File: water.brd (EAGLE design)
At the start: 100 x 80 mm, 15 parts, among them K1 AQH2223, K2 AQH2223, K3 AQH2223, K4 AQH2223, X5 MKDSN1,5/2-5,08, X6 MKDSN1,5/2-5,08, X7 MKDSN1,5/2-5,08, X8 MKDSN1,5/2-5,08

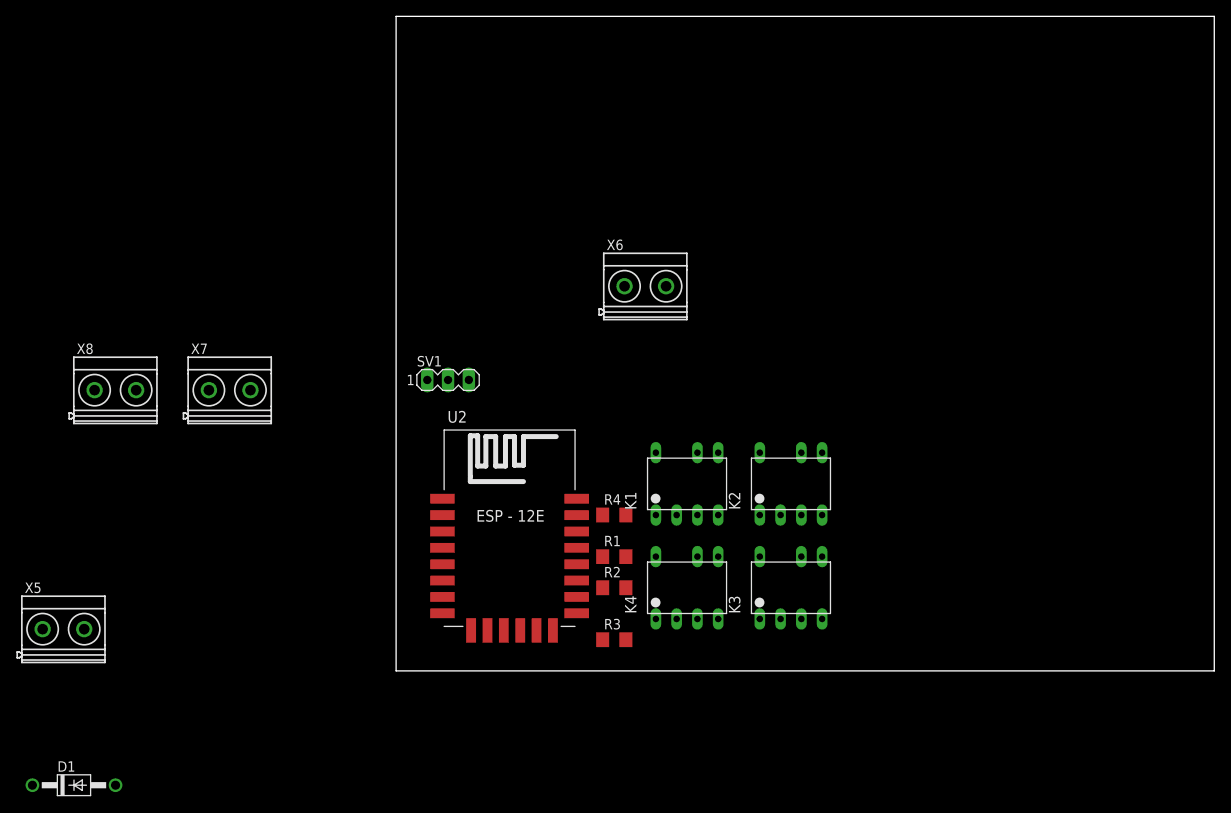
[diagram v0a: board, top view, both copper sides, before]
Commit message: Changes
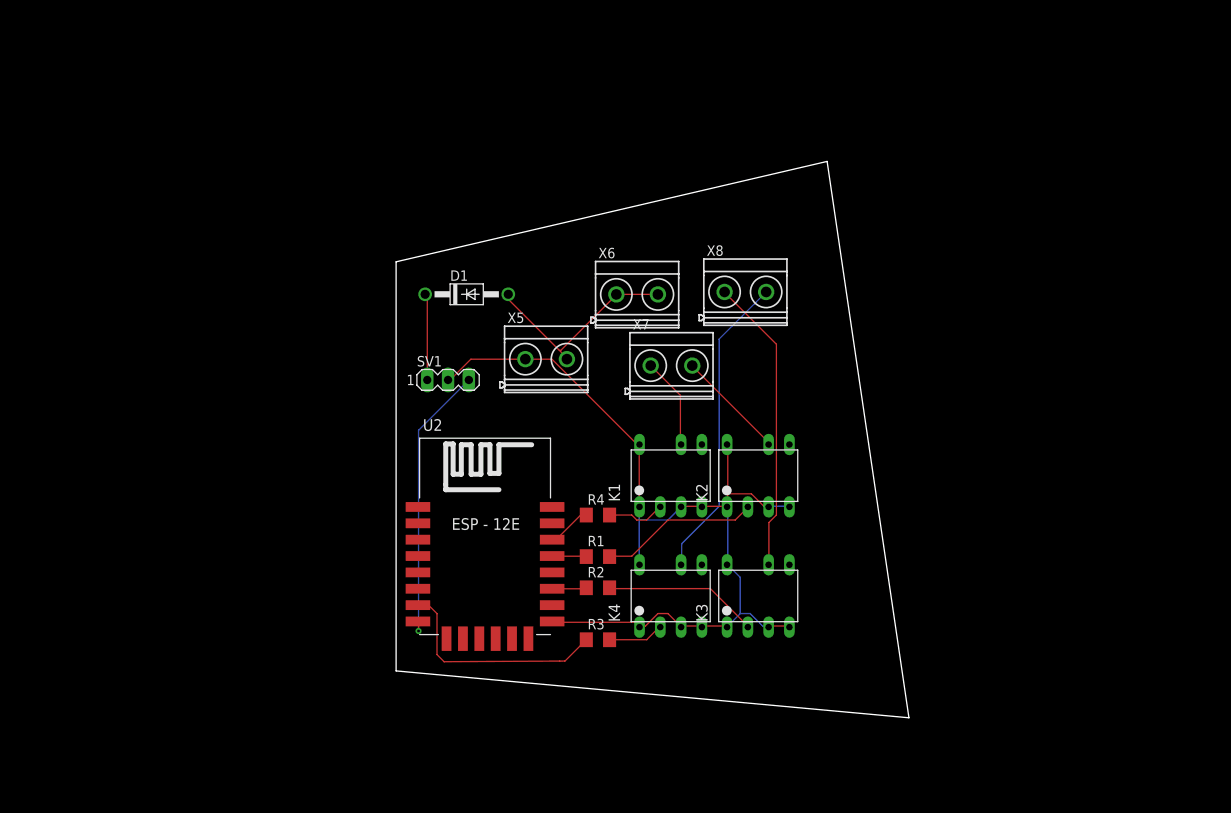
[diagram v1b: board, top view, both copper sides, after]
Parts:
- moved X8 77.9 mm to (42.7, 46.3)
- moved D1 76.8 mm to (8.63, 46.0)
- moved X5 67.6 mm to (18.4, 38.1)
- moved X7 54.1 mm to (33.7, 37.3)
- moved K2 4.12 mm to (44.3, 23.9)
- moved K3 4.12 mm to (44.3, 9.16)
- moved U2 3.16 mm to (11.0, 14.2)
- moved K1 2.24 mm to (33.6, 23.9)
- moved K4 2.24 mm to (33.6, 9.16)
- moved R1 2.00 mm to (24.7, 14.0)
- moved R2 2.00 mm to (24.7, 10.2)
- moved R3 2.00 mm to (24.7, 3.81)
- moved R4 2.00 mm to (24.7, 19.1)
- moved X6 1.41 mm to (29.5, 46.0)
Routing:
- net GND: track 0.00 -> 117.8 mm
- net N$9: track 0.00 -> 37.6 mm
- net N$10: track 0.00 -> 36.3 mm
- net +3V3: track 0.00 -> 34.4 mm, vias 0 -> 1
- net N$8: track 0.00 -> 27.5 mm
- net N$15: track 0.00 -> 25.8 mm
- net N$2: track 0.00 -> 19.4 mm
- net N$3: track 0.00 -> 19.0 mm
- net N$11: track 0.00 -> 13.5 mm
- net N$12: track 0.00 -> 11.2 mm
- net N$14: track 0.00 -> 10.6 mm
- net N$1: track 0.00 -> 7.11 mm
- net N$4: track 0.00 -> 6.83 mm
- net N$5: track 0.00 -> 5.42 mm
- net N$7: track 0.00 -> 4.23 mm
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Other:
- board size 100 x 80 mm -> 62.7 x 68 mm

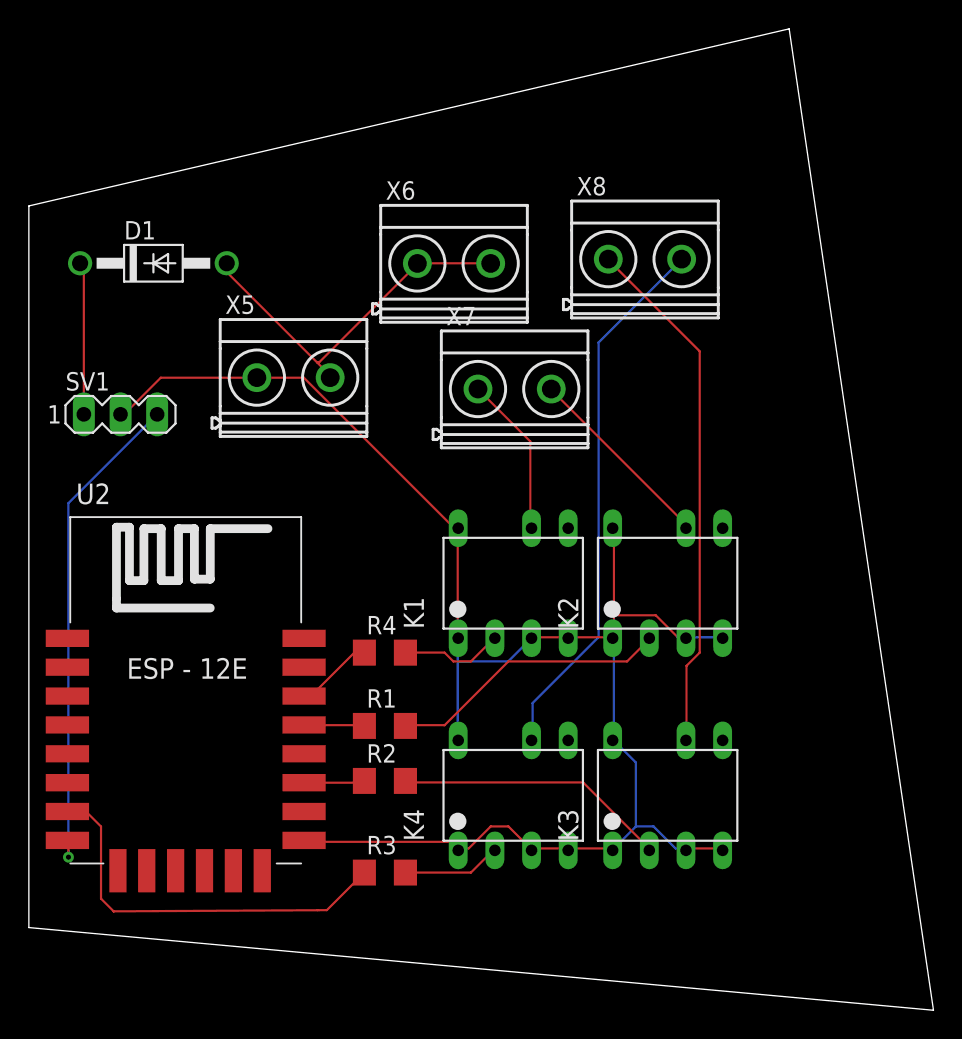
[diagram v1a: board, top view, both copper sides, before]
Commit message: Move parts
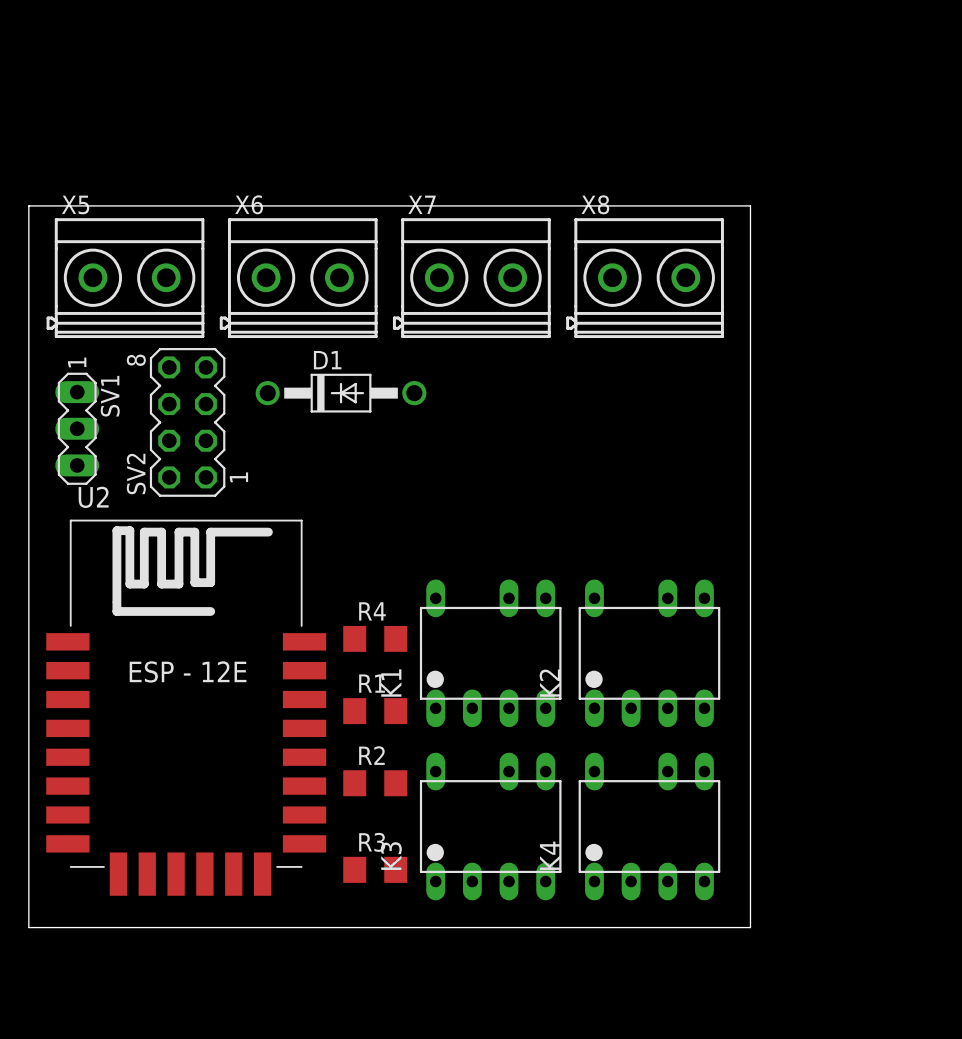
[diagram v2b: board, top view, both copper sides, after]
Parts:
- added SV2: (no value), con-lstb:MA04-2
- R1, R2, R3, R4: value 220 -> (none)
- moved D1 15.8 mm to (21.6, 37.0)
- moved X5 13.3 mm to (7.00, 45.0)
- moved K3 12.4 mm to (32.0, 7.00)
- moved X6 10.5 mm to (19.0, 45.0)
- moved K4 9.68 mm to (43.0, 7.00)
- moved X7 8.16 mm to (31.0, 45.0)
- moved K1 5.10 mm to (32.0, 19.0)
- moved K2 5.02 mm to (43.0, 19.0)
- moved SV1 3.16 mm to (3.35, 34.6), turned to 270 degrees
- moved X8 1.32 mm to (43.0, 45.0)
- moved R1 1.23 mm to (24.0, 15.0)
- moved R4 1.16 mm to (24.0, 20.0)
- moved R3 0.70 mm to (24.0, 4.00)
- moved R2 0.69 mm to (24.0, 10.0)
- moved U2 0.24 mm to (11.0, 14.0)
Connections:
- new net N$13: SV2.8, U2.CH_PD
- new net N$16: SV2.6, U2.RESET
- new net N$17: SV2.3, U2.TXD0
- new net N$18: SV2.1, U2.RXD0
- new net N$19: SV2.4, U2.GPIO15
- new net N$20: SV2.2, U2.GPIO0
- net +3V3: now also SV2.7
- net GND: now also SV2.5
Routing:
- net GND: track 117.8 -> 0.00 mm
- net N$9: track 37.6 -> 0.00 mm
- net N$10: track 36.3 -> 0.00 mm
- net +3V3: track 34.4 -> 0.00 mm, vias 1 -> 0
- net N$8: track 27.5 -> 0.00 mm
- net N$15: track 25.8 -> 0.00 mm
- net N$2: track 19.4 -> 0.00 mm
- net N$3: track 19.0 -> 0.00 mm
- net N$11: track 13.5 -> 0.00 mm
- net N$12: track 11.2 -> 0.00 mm
- net N$14: track 10.6 -> 0.00 mm
- net N$1: track 7.11 -> 0.00 mm
- net N$4: track 6.83 -> 0.00 mm
- net N$5: track 5.42 -> 0.00 mm
- net N$7: track 4.23 -> 0.00 mm
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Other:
- board size 62.7 x 68 mm -> 50 x 50 mm
